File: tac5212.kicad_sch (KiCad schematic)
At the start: 58 parts, among them J1 DIGI, J10 AIN_GND, J11 AOUT1, J12 AOUT2, J13 54-00178, J2 AIN1, J3 AOUT_GND, J4 DIN, J5 VDC, J6 Qwiic, J7 MIC_GND, J8 CLK, J9 AIN2, U1 XTAC5212IRGER, U2 SPX3819M5-L-3-3, U3 SPX3819M5-L-3-3, Y1 830207659209

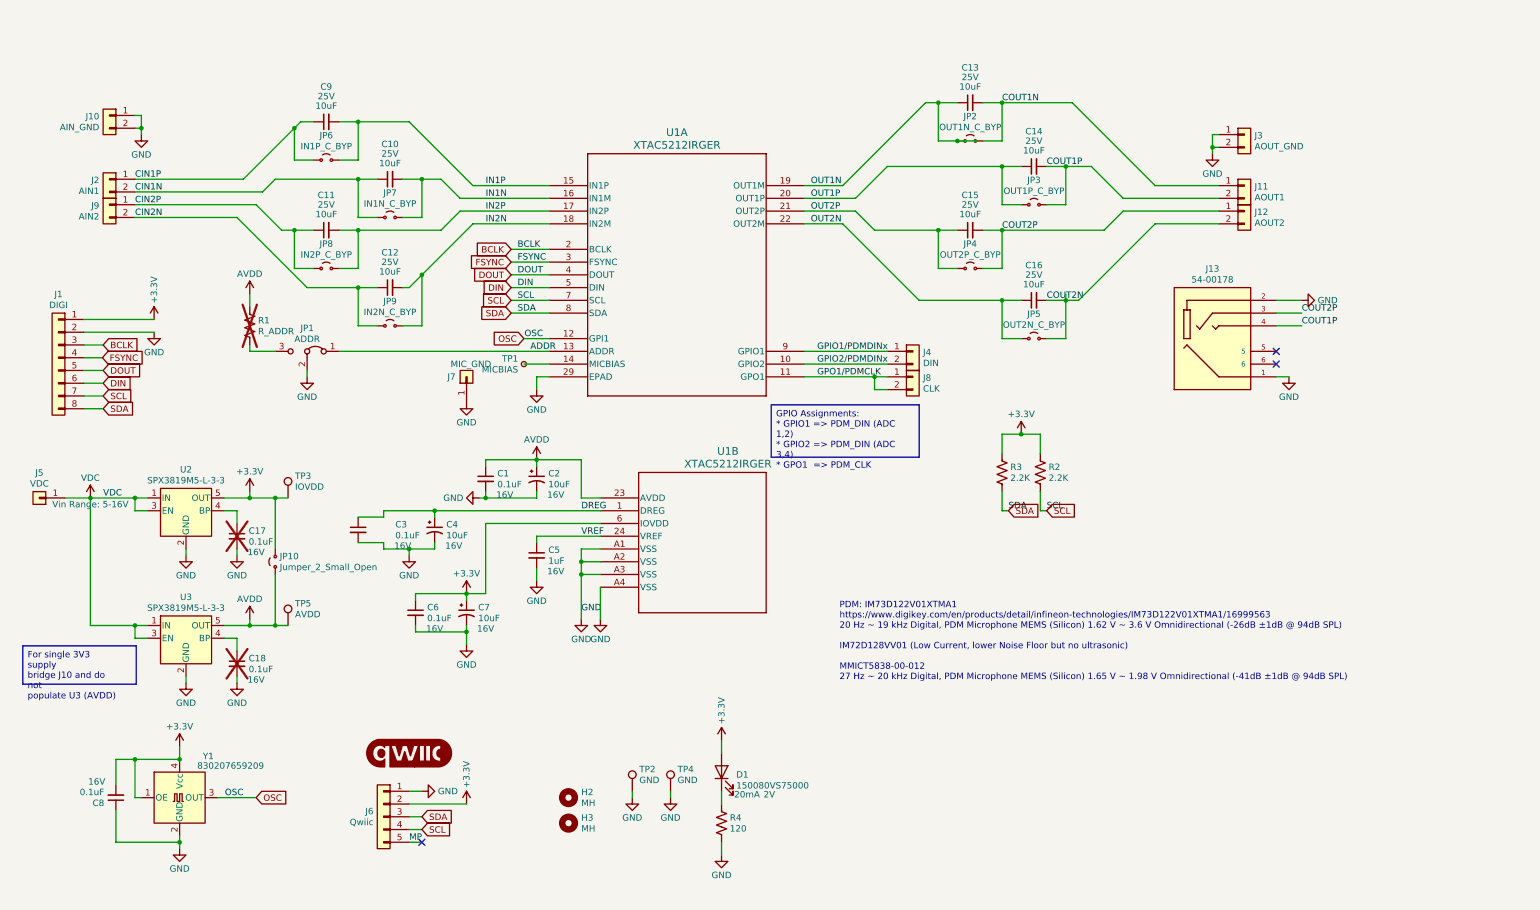
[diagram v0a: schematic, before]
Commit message: add HTML BOM
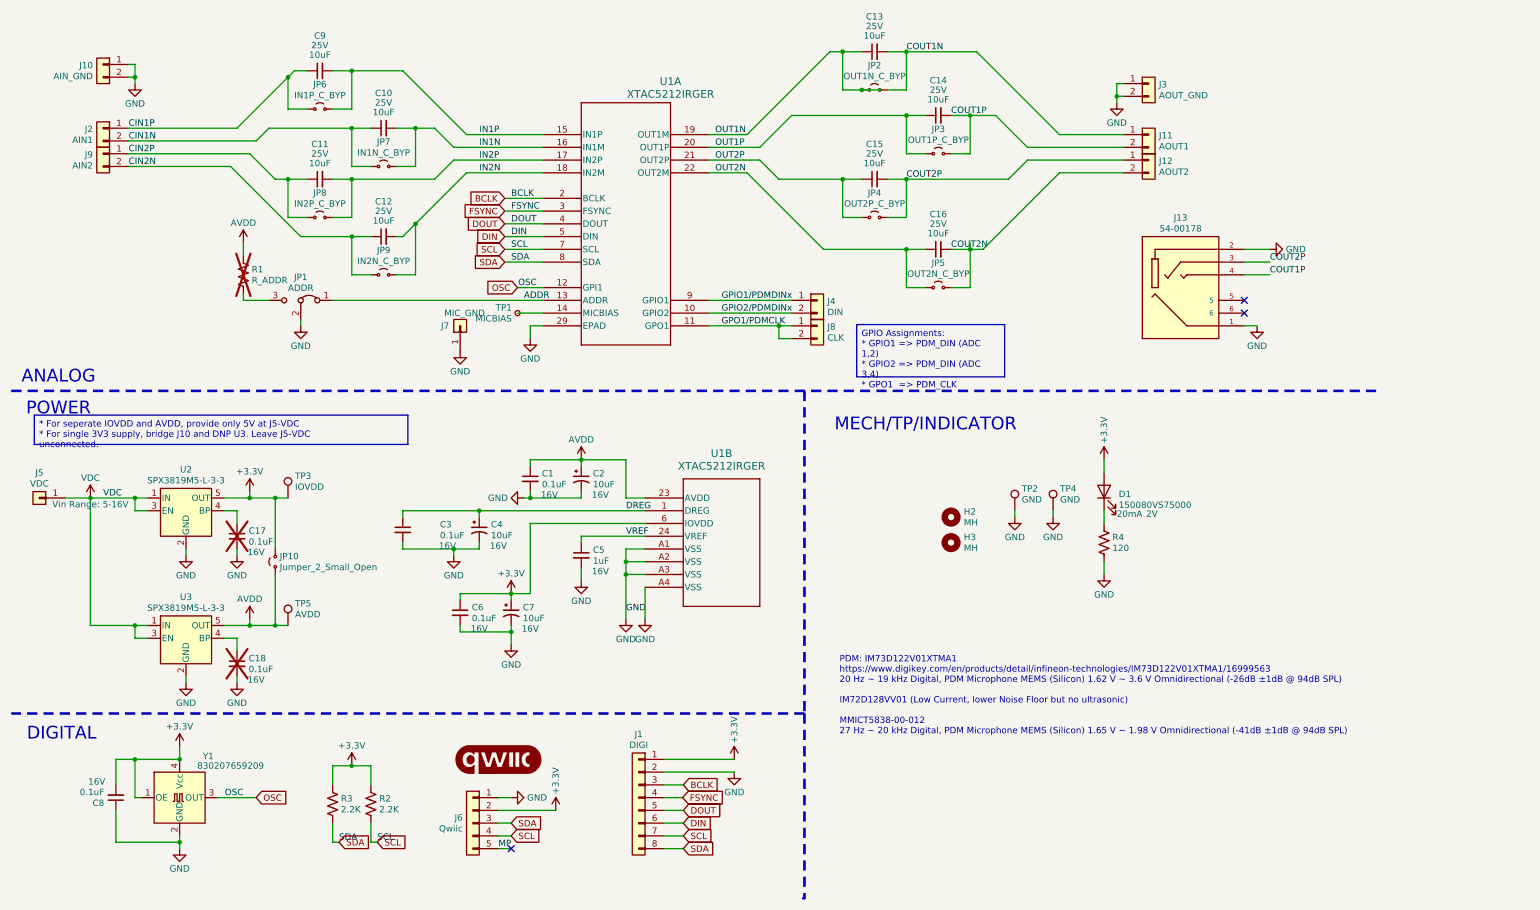
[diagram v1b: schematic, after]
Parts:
- G1, J7, JP10, TP1, TP3, TP5: now left out of the parts list
- U1: footprint footprints:VQFN24_RGE_CORNERPADS_TEX -> VQFN24_RGE_CORNERPADS_TEX
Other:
- note added: "ANALOG"
- note added: "DIGITAL"
- note added: "MECH/TP/INDICATOR"
- note added: "POWER"
- moved on the sheet: C1, C10, C11, C12, C13, C14, C15, C16, C2, C3, C4, C5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
